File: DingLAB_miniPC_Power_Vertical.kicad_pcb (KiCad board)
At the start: 2 copper layers, 33 x 22.9 mm, 8 parts, among them J1 Conn_01x02_Pin, J2 Conn_01x02_Pin, U1 KJB48xxSBO-10A

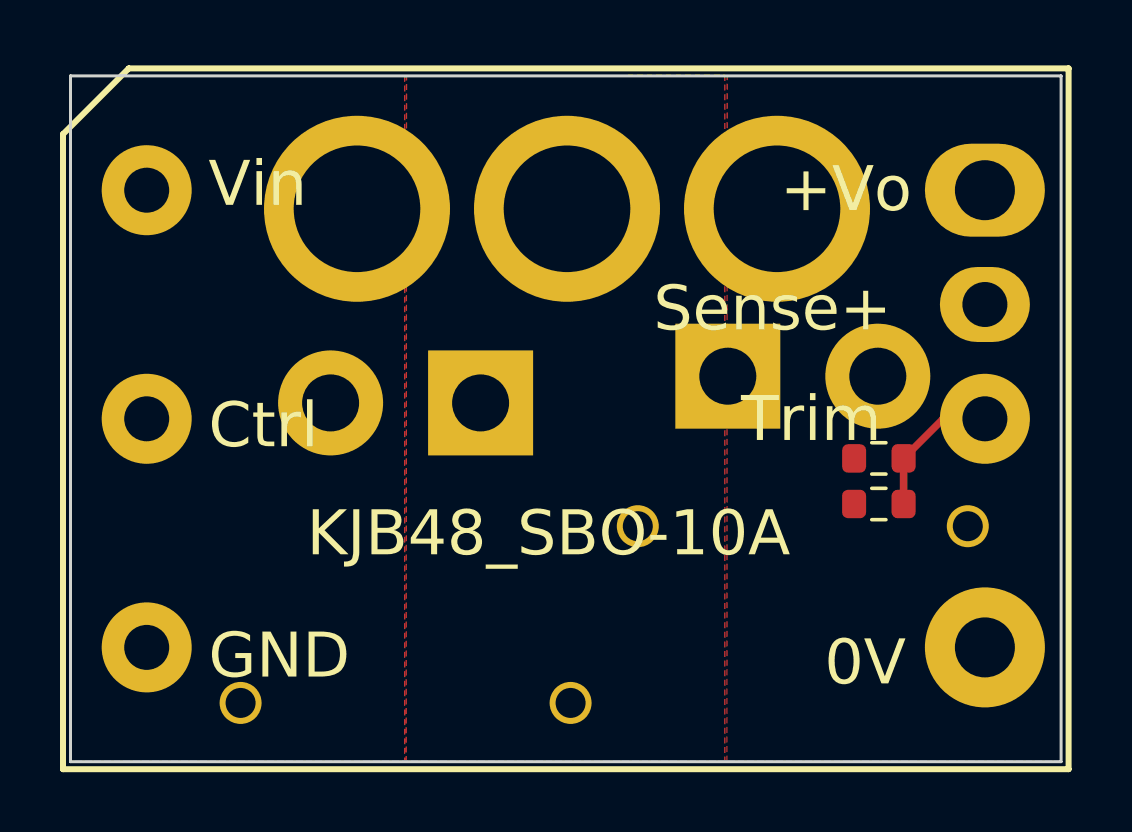
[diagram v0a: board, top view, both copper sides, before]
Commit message: Update Vertical and product
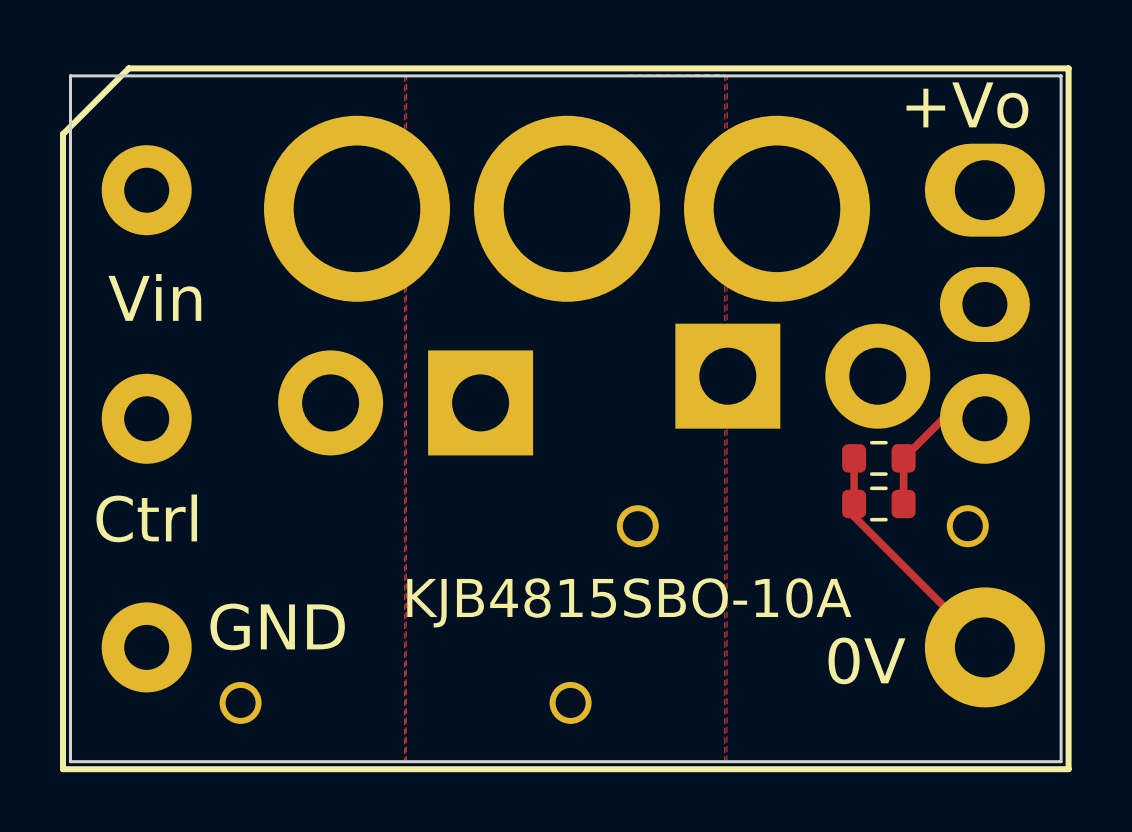
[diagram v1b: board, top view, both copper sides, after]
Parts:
- H1, H2, H3: value MountingHole -> SMTSO3060CTJ
- R1: value 150k -> 20k
- R2: value 1.15M -> ∞
- U1: value KJB48xxSBO-10A -> KJB4815SBO-10A
- turned R1 to 180 degrees
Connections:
- R1 pad 1: /Out -> Net-(U1-Trim)
- R1 pad 2: Net-(U1-Trim) -> GND
- R2 pad 1: /Out -> GND
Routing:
- net GND: track 0.00 -> 8.11 mm
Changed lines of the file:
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@@
   (net 5 "Net-(U1-Trim)")
   (footprint "Resistor_SMD:R_0603_1608Metric" (layer "F.Cu")
-    (at 126.945 114.27)
+    (at 126.945 114.27 180)
     (descr "Resistor SMD 0603 (1608 Metric), square (rectangular) end terminal, IPC_7351 nominal, (Body size source: IPC-SM-782 page 72, https://www.pcb-3d.com/wordpress/wp-content/uploads/ipc-sm-782a_amendment_1_and_2.pdf), generated with kicad-footprint-generator")
     (tags "resistor")
-    (property "Sheetfile" "DingLAB_miniPC_Power.kicad_sch")
+    (property "Sheetfile" "DingLAB_miniPC_Power_Vertical.kicad_sch")
     (property "Sheetname" "")
     (property "ki_description" "Resistor")
@@
         (effects (font (size 1 1) (thickness 0.15)))
     )
-    (fp_text value "150k" (at 0 1.43) (layer "F.Fab")
+    (fp_text value "20k" (at 0 1.43) (layer "F.Fab")
         (effects (font (size 1 1) (thickness 0.15)))
     )
@@
     (fp_line (start 0.8 0.4125) (end -0.8 0.4125)
       (stroke (width 0.1) (type solid)) (layer "F.Fab"))
-    (pad "1" smd roundrect (at -0.825 0) (size 0.8 0.95) (layers "F.Cu" "F.Paste" "F.Mask") (roundrect_rratio 0.25)
-      (net 3 "/Out") (pintype "passive"))
-    (pad "2" smd roundrect (at 0.825 0) (size 0.8 0.95) (layers "F.Cu" "F.Paste" "F.Mask") (roundrect_rratio 0.25)
+    (pad "1" smd roundrect (at -0.825 0 180) (size 0.8 0.95) (layers "F.Cu" "F.Paste" "F.Mask") (roundrect_rratio 0.25)
       (net 5 "Net-(U1-Trim)") (pintype "passive"))
+    (pad "2" smd roundrect (at 0.825 0 180) (size 0.8 0.95) (layers "F.Cu" "F.Paste" "F.Mask") (roundrect_rratio 0.25)
+      (net 2 "GND") (pintype "passive"))
     (model "${KICAD6_3DMODEL_DIR}/Resistor_SMD.3dshapes/R_0603_1608Metric.wrl"
       (offset (xyz 0 0 0))
@@
     (descr "Resistor SMD 0603 (1608 Metric), square (rectangular) end terminal, IPC_7351 nominal, (Body size source: IPC-SM-782 page 72, https://www.pcb-3d.com/wordpress/wp-content/uploads/ipc-sm-782a_amendment_1_and_2.pdf), generated with kicad-footprint-generator")
     (tags "resistor")
-    (property "Sheetfile" "DingLAB_miniPC_Power.kicad_sch")
+    (property "Sheetfile" "DingLAB_miniPC_Power_Vertical.kicad_sch")
     (property "Sheetname" "")
     (property "ki_description" "Resistor")
@@
         (effects (font (size 1 1) (thickness 0.15)))
     )
-    (fp_text value "1.15M" (at 0 1.43) (layer "F.Fab")
+    (fp_text value "∞" (at 0 1.43) (layer "F.Fab")
         (effects (font (size 1 1) (thickness 0.15)))
     )
@@
       (stroke (width 0.1) (type solid)) (layer "F.Fab"))
     (pad "1" smd roundrect (at -0.825 0) (size 0.8 0.95) (layers "F.Cu" "F.Paste" "F.Mask") (roundrect_rratio 0.25)
-      (net 3 "/Out") (pintype "passive"))
+      (net 2 "GND") (pintype "passive"))
     (pad "2" smd roundrect (at 0.825 0) (size 0.8 0.95) (layers "F.Cu" "F.Paste" "F.Mask") (roundrect_rratio 0.25)
       (net 5 "Net-(U1-Trim)") (pintype "passive"))
@@
   (footprint "DingLAB_miniPC_Power:KJB48_SBO-10A" (layer "F.Cu")
     (at 116.51 111.43)
-    (property "Sheetfile" "DingLAB_miniPC_Power.kicad_sch")
+    (property "Sheetfile" "DingLAB_miniPC_Power_Vertical.kicad_sch")
     (property "Sheetname" "")
     (fp_text reference "U1" (at 0 0) (layer "F.SilkS") hide
         (effects (font (size 1.27 1.27) (thickness 0.15)))
     )
-    (fp_text value "KJB48xxSBO-10A" (at 0 10.033) (layer "F.SilkS") hide
+    (fp_text value "KJB4815SBO-10A" (at 2.04 6.02) (layer "F.SilkS")
         (effects (font (size 1.27 1.27) (thickness 0.15)))
     )
-    (fp_text user "Vin" (at -11.9125 -6.94726 unlocked) (layer "F.SilkS")
-        (effects (font (size 1.5 1.5) (thickness 0.3048)) (justify left bottom))
-    )
-    (fp_text user "Ctrl" (at -11.90973 1.09699 unlocked) (layer "F.SilkS")
-        (effects (font (size 1.5 1.5) (thickness 0.3048)) (justify left bottom))
-    )
-    (fp_text user "KJB48_SBO-10A" (at -8.636 4.699 unlocked) (layer "F.SilkS")
-        (effects (font (size 1.5 1.5) (thickness 0.3048)) (justify left bottom))
-    )
-    (fp_text user "+Vo" (at 7.14514 -6.77287 unlocked) (layer "F.SilkS")
-        (effects (font (size 1.5 1.5) (thickness 0.3048)) (justify left bottom))
-    )
-    (fp_text user "GND" (at -11.90973 8.7756 unlocked) (layer "F.SilkS")
-        (effects (font (size 1.5 1.5) (thickness 0.3048)) (justify left bottom))
-    )
-    (fp_text user "Sense+" (at 2.921 -2.794 unlocked) (layer "F.SilkS")
+    (fp_text user "Vin" (at -15.26 -3.08 unlocked) (layer "F.SilkS")
+        (effects (font (size 1.5 1.5) (thickness 0.3048)) (justify left bottom))
+    )
+    (fp_text user "Ctrl" (at -15.76 4.27 unlocked) (layer "F.SilkS")
+        (effects (font (size 1.5 1.5) (thickness 0.3048)) (justify left bottom))
+    )
+    (fp_text user "KJB48_SBO-10A" (at -8.636 4.699 unlocked) (layer "F.SilkS") hide
+        (effects (font (size 1.5 1.5) (thickness 0.3048)) (justify left bottom))
+    )
+    (fp_text user "+Vo" (at 11.14 -9.53 unlocked) (layer "F.SilkS")
+        (effects (font (size 1.5 1.5) (thickness 0.3048)) (justify left bottom))
+    )
+    (fp_text user "GND" (at -11.96 7.87 unlocked) (layer "F.SilkS")
         (effects (font (size 1.5 1.5) (thickness 0.3048)) (justify left bottom))
     )
     (fp_text user "0V" (at 8.62209 9.00223 unlocked) (layer "F.SilkS")
-        (effects (font (size 1.5 1.5) (thickness 0.3048)) (justify left bottom))
-    )
-    (fp_text user "Trim" (at 5.842 0.889 unlocked) (layer "F.SilkS")
         (effects (font (size 1.5 1.5) (thickness 0.3048)) (justify left bottom))
     )
@@
   (footprint "DingLAB_miniPC_Power:SMTSO3060CTJ" (layer "B.Cu")
     (at 123.55 104.43 180)
-    (property "Sheetfile" "DingLAB_miniPC_Power.kicad_sch")
+    (property "Sheetfile" "DingLAB_miniPC_Power_Vertical.kicad_sch")
     (property "Sheetname" "")
     (property "ki_description" "Mounting Hole without connection")
     (property "ki_keywords" "mounting hole")
+    (property "lcsc" "C2915637")
     (attr smd)
-    (fp_text reference "H2" (at 0 4.064 unlocked) (layer "B.SilkS")
+    (fp_text reference "H2" (at 0 4.064 unlocked) (layer "B.SilkS") hide
         (effects (font (size 1 1) (thickness 0.1)) (justify mirror))
     )
-    (fp_text value "MountingHole" (at 0 -4.215 unlocked) (layer "B.Fab")
+    (fp_text value "SMTSO3060CTJ" (at 0 -4.215 unlocked) (layer "B.Fab")
         (effects (font (size 1 1) (thickness 0.15)) (justify mirror))
     )
@@
   (footprint "DingLAB_miniPC_Power:SMTSO3060CTJ" (layer "B.Cu")
     (at 109.55 104.43 180)
-    (property "Sheetfile" "DingLAB_miniPC_Power.kicad_sch")
+    (property "Sheetfile" "DingLAB_miniPC_Power_Vertical.kicad_sch")
     (property "Sheetname" "")
     (property "ki_description" "Mounting Hole without connection")
     (property "ki_keywords" "mounting hole")
+    (property "lcsc" "C2915637")
     (attr smd)
-    (fp_text reference "H3" (at 0 4.064 unlocked) (layer "B.SilkS")
+    (fp_text reference "H3" (at 0 4.064 unlocked) (layer "B.SilkS") hide
         (effects (font (size 1 1) (thickness 0.1)) (justify mirror))
     )
-    (fp_text value "MountingHole" (at 0 -4.215 unlocked) (layer "B.Fab")
+    (fp_text value "SMTSO3060CTJ" (at 0 -4.215 unlocked) (layer "B.Fab")
         (effects (font (size 1 1) (thickness 0.15)) (justify mirror))
     )
@@
   (footprint "DingLAB_miniPC_Power:SMTSO3060CTJ" (layer "B.Cu")
     (at 116.55 104.43 180)
-    (property "Sheetfile" "DingLAB_miniPC_Power.kicad_sch")
+    (property "Sheetfile" "DingLAB_miniPC_Power_Vertical.kicad_sch")
     (property "Sheetname" "")
     (property "ki_description" "Mounting Hole without connection")
     (property "ki_keywords" "mounting hole")
+    (property "lcsc" "C2915637")
     (attr smd)
     (fp_text reference "H1" (at 0 4.064 unlocked) (layer "B.SilkS") hide
         (effects (font (size 1 1) (thickness 0.1)) (justify mirror))
     )
-    (fp_text value "MountingHole" (at 0 -4.215 unlocked) (layer "B.Fab")
+    (fp_text value "SMTSO3060CTJ" (at 0 -4.215 unlocked) (layer "B.Fab")
         (effects (font (size 1 1) (thickness 0.15)) (justify mirror))
     )
@@
     (descr "Connector XT30 Horizontal PCB Female, https://www.tme.eu/en/Document/ce4077e36b79046da520ca73227e15de/XT30PW%20SPEC.pdf")
     (tags "RC Connector XT30")
-    (property "Sheetfile" "DingLAB_miniPC_Power.kicad_sch")
+    (property "Sheetfile" "DingLAB_miniPC_Power_Vertical.kicad_sch")
     (property "Sheetname" "")
     (property "ki_description" "Generic connector, single row, 01x02, script generated")
@@
         (effects (font (size 1 1) (thickness 0.15)) (justify mirror))
     )
-    (fp_text user "+" (at 8 0) (layer "B.SilkS")
+    (fp_text user "+" (at 4.99 2.89) (layer "B.SilkS")
         (effects (font (size 1.5 1.5) (thickness 0.15)) (justify mirror))
     )
@@
     (descr "Connector XT30 Horizontal PCB Male, https://www.tme.eu/en/Document/ce4077e36b79046da520ca73227e15de/XT30PW%20SPEC.pdf")
     (tags "RC Connector XT30")
-    (property "Sheetfile" "DingLAB_miniPC_Power.kicad_sch")
+    (property "Sheetfile" "DingLAB_miniPC_Power_Vertical.kicad_sch")
     (property "Sheetname" "")
     (property "ki_description" "Generic connector, single row, 01x02, script generated")
@@
   (gr_rect (start 100 100) (end 133.02 122.86)
     (stroke (width 0.1) (type default)) (fill none) (layer "Edge.Cuts"))
+  (segment (start 126.12 114.69) (end 130.48 119.05) (width 0.25) (layer "F.Cu") (net 2))
+  (segment (start 126.12 112.75) (end 126.12 114.27) (width 0.25) (layer "F.Cu") (net 2))
+  (segment (start 126.12 114.27) (end 126.12 114.69) (width 0.25) (layer "F.Cu") (net 2))
   (segment (start 130.48 111.43) (end 129.09 111.43) (width 0.25) (layer "F.Cu") (net 5))
   (segment (start 127.77 112.75) (end 127.77 114.27) (width 0.25) (layer "F.Cu") (net 5))

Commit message: Fix bug
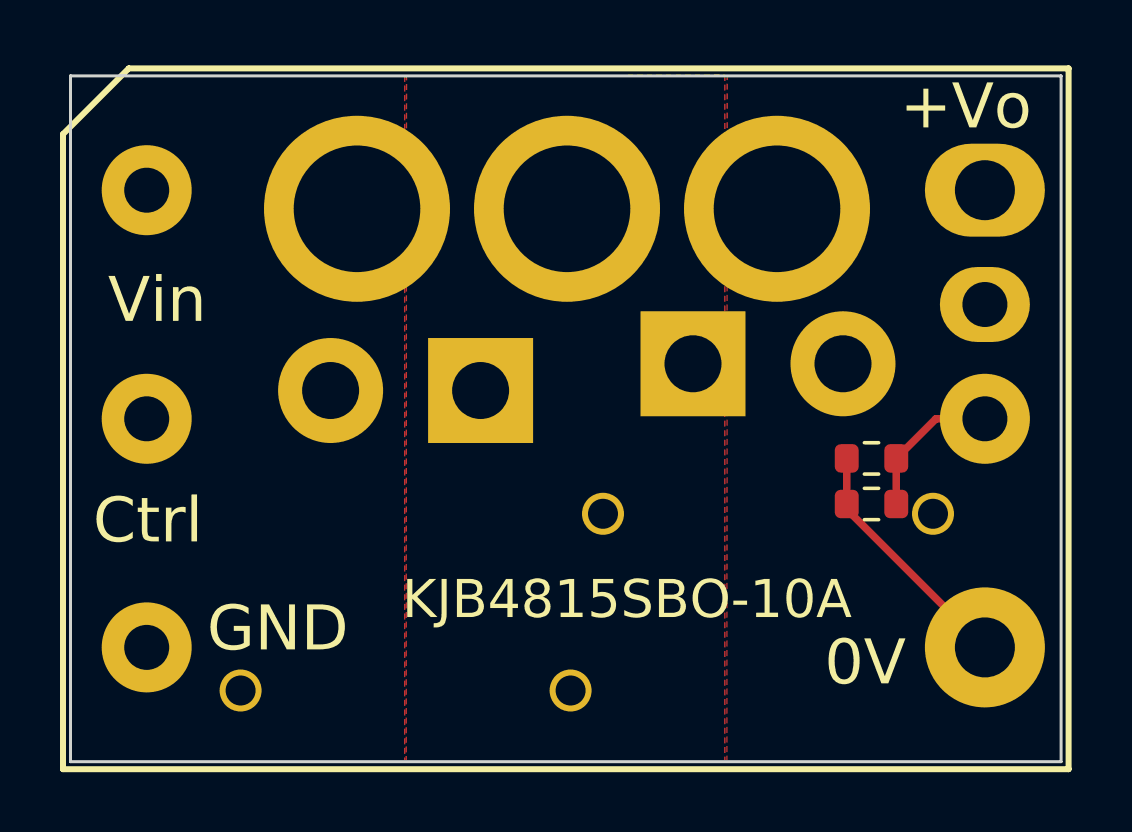
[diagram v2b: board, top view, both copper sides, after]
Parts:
- moved J1 1.23 mm to (120.8, 109.6)
- moved J2 0.41 mm to (113.7, 110.5)
- moved R1 0.24 mm to (126.7, 114.3)
- moved R2 0.24 mm to (126.7, 112.8)
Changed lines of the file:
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@@
   (net 5 "Net-(U1-Trim)")
   (footprint "Resistor_SMD:R_0603_1608Metric" (layer "F.Cu")
-    (at 126.945 114.27 180)
+    (at 126.7 114.27 180)
     (descr "Resistor SMD 0603 (1608 Metric), square (rectangular) end terminal, IPC_7351 nominal, (Body size source: IPC-SM-782 page 72, https://www.pcb-3d.com/wordpress/wp-content/uploads/ipc-sm-782a_amendment_1_and_2.pdf), generated with kicad-footprint-generator")
     (tags "resistor")
@@
   )
   (footprint "Resistor_SMD:R_0603_1608Metric" (layer "F.Cu")
-    (at 126.945 112.75)
+    (at 126.7 112.75)
     (descr "Resistor SMD 0603 (1608 Metric), square (rectangular) end terminal, IPC_7351 nominal, (Body size source: IPC-SM-782 page 72, https://www.pcb-3d.com/wordpress/wp-content/uploads/ipc-sm-782a_amendment_1_and_2.pdf), generated with kicad-footprint-generator")
     (tags "resistor")
@@
   )
   (footprint "DingLAB_miniPC_Power:AMASS_XT30PW-F_Horizontal" (layer "B.Cu")
-    (at 121.91 110.01)
+    (at 120.75 109.596)
     (descr "Connector XT30 Horizontal PCB Female, https://www.tme.eu/en/Document/ce4077e36b79046da520ca73227e15de/XT30PW%20SPEC.pdf")
     (tags "RC Connector XT30")
@@
   )
   (footprint "DingLAB_miniPC_Power:AMASS_XT30PW-M_Horizontal" (layer "B.Cu")
-    (at 113.67 110.901)
+    (at 113.67 110.487)
     (descr "Connector XT30 Horizontal PCB Male, https://www.tme.eu/en/Document/ce4077e36b79046da520ca73227e15de/XT30PW%20SPEC.pdf")
     (tags "RC Connector XT30")
@@
   (gr_rect (start 100 100) (end 133.02 122.86)
     (stroke (width 0.1) (type default)) (fill none) (layer "Edge.Cuts"))
-  (segment (start 126.12 114.69) (end 130.48 119.05) (width 0.25) (layer "F.Cu") (net 2))
-  (segment (start 126.12 112.75) (end 126.12 114.27) (width 0.25) (layer "F.Cu") (net 2))
-  (segment (start 126.12 114.27) (end 126.12 114.69) (width 0.25) (layer "F.Cu") (net 2))
-  (segment (start 130.48 111.43) (end 129.09 111.43) (width 0.25) (layer "F.Cu") (net 5))
-  (segment (start 127.77 112.75) (end 127.77 114.27) (width 0.25) (layer "F.Cu") (net 5))
-  (segment (start 129.09 111.43) (end 127.77 112.75) (width 0.25) (layer "F.Cu") (net 5))
+  (segment (start 125.875 112.75) (end 125.875 114.27) (width 0.25) (layer "F.Cu") (net 2))
+  (segment (start 125.875 114.445) (end 130.48 119.05) (width 0.25) (layer "F.Cu") (net 2))
+  (segment (start 125.875 114.27) (end 125.875 114.445) (width 0.25) (layer "F.Cu") (net 2))
+  (segment (start 127.525 112.75) (end 127.525 114.27) (width 0.25) (layer "F.Cu") (net 5))
+  (segment (start 130.48 111.43) (end 128.845 111.43) (width 0.25) (layer "F.Cu") (net 5))
+  (segment (start 128.845 111.43) (end 127.525 112.75) (width 0.25) (layer "F.Cu") (net 5))
   (zone (net 3) (net_name "/Out") (layer "F.Cu") (hatch edge 0.5)
     (priority 1)

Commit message: Update
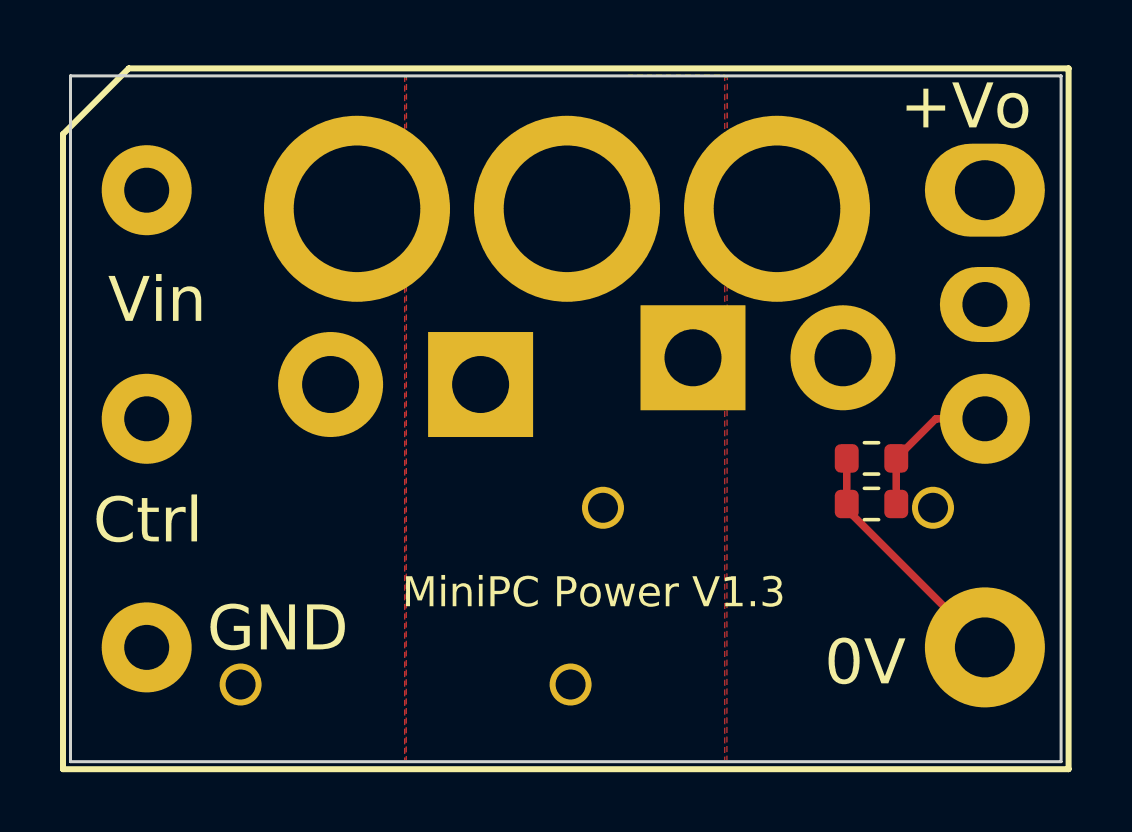
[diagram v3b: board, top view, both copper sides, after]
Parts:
- moved J1 0.20 mm to (120.8, 109.4)
- moved J2 0.20 mm to (113.7, 110.3)
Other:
- board text added: "MiniPC Power V1.3"
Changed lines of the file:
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@@
         (effects (font (size 1.27 1.27) (thickness 0.15)))
     )
-    (fp_text value "KJB4815SBO-10A" (at 2.04 6.02) (layer "F.SilkS")
+    (fp_text value "KJB4815SBO-10A" (at 2.04 6.02) (layer "F.SilkS") hide
         (effects (font (size 1.27 1.27) (thickness 0.15)))
     )
@@
   )
   (footprint "DingLAB_miniPC_Power:AMASS_XT30PW-F_Horizontal" (layer "B.Cu")
-    (at 120.75 109.596)
+    (at 120.75 109.396)
     (descr "Connector XT30 Horizontal PCB Female, https://www.tme.eu/en/Document/ce4077e36b79046da520ca73227e15de/XT30PW%20SPEC.pdf")
     (tags "RC Connector XT30")
@@
   )
   (footprint "DingLAB_miniPC_Power:AMASS_XT30PW-M_Horizontal" (layer "B.Cu")
-    (at 113.67 110.487)
+    (at 113.67 110.287)
     (descr "Connector XT30 Horizontal PCB Male, https://www.tme.eu/en/Document/ce4077e36b79046da520ca73227e15de/XT30PW%20SPEC.pdf")
     (tags "RC Connector XT30")
@@
   (gr_rect (start 100 100) (end 133.02 122.86)
     (stroke (width 0.1) (type default)) (fill none) (layer "Edge.Cuts"))
+  (gr_text "MiniPC Power V1.3" (at 111.05 117.8) (layer "F.SilkS")
+    (effects (font (size 1 1) (thickness 0.15)) (justify left bottom))
+  )
   (segment (start 125.875 112.75) (end 125.875 114.27) (width 0.25) (layer "F.Cu") (net 2))
   (segment (start 125.875 114.445) (end 130.48 119.05) (width 0.25) (layer "F.Cu") (net 2))
